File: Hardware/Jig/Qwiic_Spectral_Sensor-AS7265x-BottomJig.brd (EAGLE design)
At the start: 35.6 x 40.6 mm, 93 parts, among them J2 Serial Interface, J5 Flash Programming, J8 PTH, U1 AS72651, U3 4MB Flash, U5 AS72653, U6 AS72652

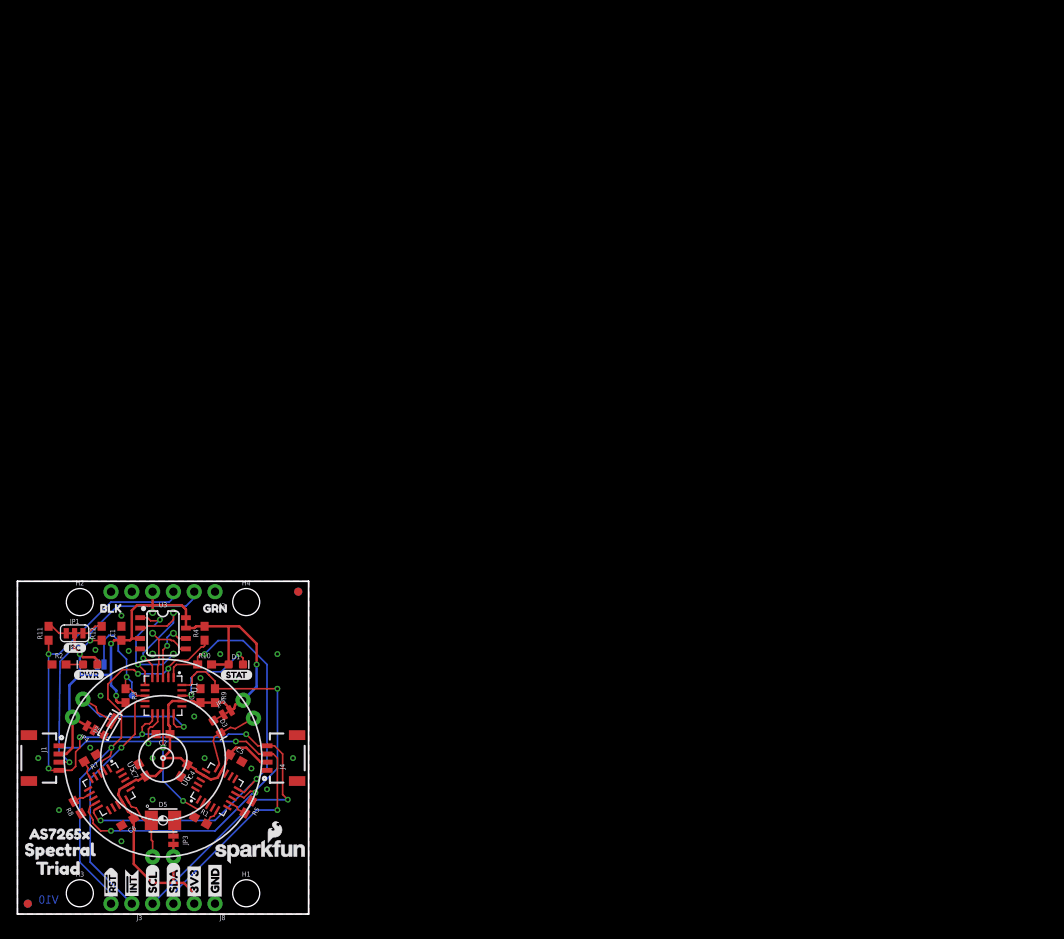
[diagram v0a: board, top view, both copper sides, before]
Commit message: Silk changes before panelization
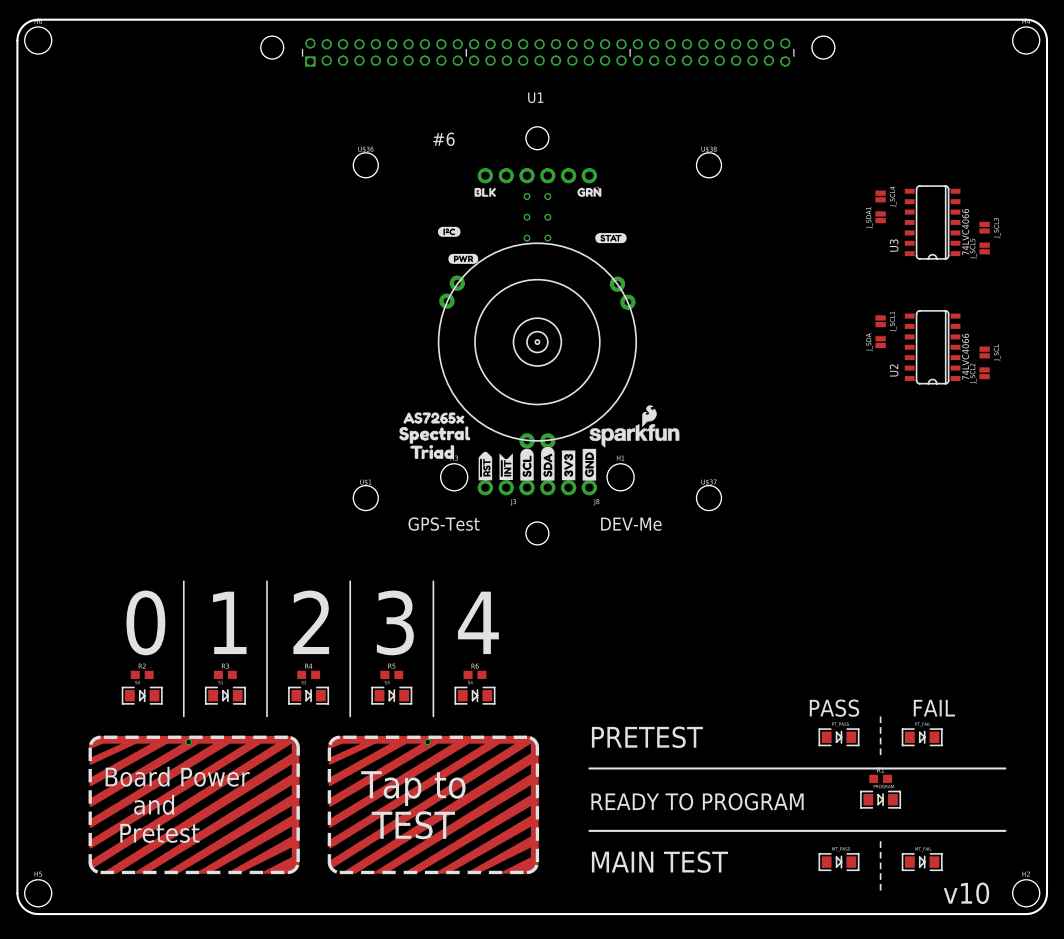
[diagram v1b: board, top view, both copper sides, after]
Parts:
- removed C1: 1.0uF, SparkFun-Capacitors:0603
- removed C2, C4, C6: 0.1uF, SparkFun-Capacitors:0603
- removed C3, C5, C7: 10uF, SparkFun-Capacitors:0603
- removed D1: BLUE, SparkFun-LED:LED-0603
- removed D2: 5700k, SparkFun-LED:SUPER_BRIGHT_SMD_LED_3014
- removed D3: IR, SparkFun-LED:LED-0603
- removed D4: RED, SparkFun-LED:LED-0603
- removed D5: UV, SparkFun-LED:PLCC-2
- removed FD1, FD2, FD3, FD4: FIDUCIAL1X2, SparkFun-Aesthetics:FIDUCIAL-1X2
- removed J1, J4: (no value), SparkFun-Connectors:1X04_1MM_RA
- removed JP1: (no value), SparkFun-Jumpers:SMT-JUMPER_3_2-NC_TRACE_SILK
- removed JP2: (no value), SparkFun-Jumpers:SMT-JUMPER_2_NO_SILK
- removed JP3, JP4, JP5: (no value), SparkFun-Jumpers:SMT-JUMPER_2_NC_TRACE_NO-SILK
- removed R10, R11, R12, R9: 2.2k, SparkFun-Resistors:0603
- removed R7, R8: 10k, SparkFun-Resistors:0603
- removed TP1: (no value), SparkFun-Connectors:PAD.03X.03
- removed U5: AS72653, Qwiic_Spectral_Sensor-AS7265x:LGA20
- removed U6: AS72652, Qwiic_Spectral_Sensor-AS7265x:LGA20
- added BUTTON1, BUTTON2: CAPSENSE_BUTTON_PAD_ONLY, Testing:CAPSENSE_BUTTON_PADS_ONLY
- added FRAME2: FRAME-LEDGER, SparkFun-Aesthetics:CREATIVE_COMMONS
- added H5, H6: STAND-OFF, SparkFun-Hardware:STAND-OFF
- added J_SCL, J_SCL3, J_SDA, J_SDA1: JUMPER-SMT_2_NO_NO-SILK, SparkFun-Jumpers:SMT-JUMPER_2_NO_NO-SILK
- added J_SCL1, J_SCL2, J_SCL4, J_SCL5: (no value), SparkFun-Jumpers:SMT-JUMPER_2_NO_NO-SILK
- added MT_FAIL, MT_PASS, PROGRAM, PT_FAIL, PT_PASS, S0, S1, S2, S3, S4: (no value), Testing:LED-1206
- added R6: 330, SparkFun-Resistors:0603
- added U2: 74LVC4066, Testing:SO14
- R1, R3, R4, R5: value 10k -> 330
- R2: value 1k -> 330
- U$1, U$36, U$37: device buzzard_labels (7):#0 -> SparkFun-Hardware:STAND-OFF-TIGHT
- U$38: device buzzard_labels (7):#1 -> SparkFun-Hardware:STAND-OFF-TIGHT
- U$39, U$40: device buzzard_labels (7):#1 -> SparkFun-Hardware:NUBBIN_LOCKER
- U1: value AS72651 -> FLYING_JALAPENO; device Qwiic_Spectral_Sensor-AS7265x:LGA20 -> Testing:FLYING_JALAPENO_V3_M
- U3: value 4MB Flash -> 74LVC4066; device SparkFun-IC-Memory:SO08 -> Testing:SO14
- moved H2 120.9 mm to (123.2, 2.54)
- moved H4 117.4 mm to (123.2, 106.7)
- moved U$38 108.9 mm to (84.5, 91.4), flipped to the top
- moved U3 106.2 mm to (111.8, 83.8), turned to 90 degrees
- moved U1 95.0 mm to (64.8, 109.2), turned to 0 degrees
- moved R1 83.2 mm to (105.4, 16.5), turned to 0 degrees
- moved U$40 78.1 mm to (63.5, 94.7), flipped to the top, turned to 0 degrees
- moved U$37 76.6 mm to (84.5, 50.8), flipped to the top
- moved U$36 74.8 mm to (42.5, 91.4), flipped to the top, turned to 0 degrees
- moved U$6 70.6 mm to (70.6, 77.5), turned to 240 degrees
- moved U$10 70.3 mm to (70.5, 82.5)
- moved BULB2 68.3 mm to (73.9, 75.8)
- moved BULB3 68.3 mm to (63.5, 57.8)
- moved H3 68.3 mm to (53.3, 53.3)
- moved J5 68.3 mm to (63.5, 85.1)
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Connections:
- removed net !RST-ADDR: U1.13, U6.2
- removed net I2C_ENB: JP2.2, R3.1, TP1.P$1, U1.8
- removed net N$1: D4.C, R2.2
- removed net N$11: D5.A, JP3.1
- removed net N$12: R8.2, U5.7
- removed net N$13: R7.2, U5.5
- removed net N$2: D1.C, U1.18
- removed net N$3: R5.2, U6.7
- removed net N$4: JP1.3, R12.2
- removed net N$5: JP1.1, R11.2
- removed net N$6: D2.A, JP4.1
- removed net N$8: D3.A, JP5.1
- removed net N$9: R1.2, U6.5
- removed net SCL_S: R9.1, U1.20, U5.9, U6.9
- removed net SDA_S: R10.1, U1.1, U5.10, U6.10
- new net 3.3V_POWER: U1.2, U1.32, U2.14, U3.14
- new net 5V_POWER: U1.3, U1.33
- new net JALAPENO_CS: J_SDA1.1, U1.60, U3.11
- new net JALAPENO_I2C_EN: U1.24, U2.13, U2.5
- new net JALAPENO_MISO: J_SCL5.1, U1.29, U3.1
- new net JALAPENO_MOSI: J_SCL3.1, U1.59, U3.4
- new net JALAPENO_RX1-I: J_SDA.1, U1.52, U2.11
- new net JALAPENO_SCK: J_SCL4.1, U1.30, U3.8
- new net JALAPENO_SCL: J_SCL.1, U1.53, U2.4
- new net JALAPENO_SDA: J_SCL2.1, U1.23, U2.1
- new net JALAPENO_SERIAL_EN: U1.54, U2.12, U2.6
- new net JALAPENO_SPI_EN: U3.12, U3.13, U3.5, U3.6
- new net JALAPENO_TX1-O: J_SCL1.1, U1.22, U2.8
- new net J_24: U1.25
- new net J_25: U1.55
- new net J_26: U1.26
- new net J_27: U1.56
- new net J_28: U1.27
- new net J_29: U1.57
- new net J_30: U1.28
- new net J_A0: U1.37
- new net J_A1: U1.8
- new net J_A2: U1.38
- new net J_A3: U1.9
- new net J_A4: U1.39
- new net J_PWM2: U1.14
- new net J_PWM3: U1.44
- new net J_PWM4: U1.15
- new net J_PWM5: U1.45
- new net N$10: PT_FAIL.A, U1.36
- new net N$14: MT_PASS.A, U1.6
- new net N$15: MT_FAIL.A, U1.35
- new net N$16: BUTTON2.CAPSENSE_PAD, U1.58
- new net N$17: BUTTON1.CAPSENSE_PAD, U1.5
- new net N$18: R1.2, U1.19
- new net N$19: PROGRAM.A, R1.1
- new net N$20: R6.2, U1.46
- new net N$21: R5.2, U1.17
- new net N$22: R4.2, U1.47
- new net N$23: R3.2, U1.18
- new net N$24: R2.2, U1.48
- new net N$25: R6.1, S4.A
- new net N$26: R5.1, S3.A
- new net N$27: R4.1, S2.A
- new net N$28: R3.1, S1.A
- new net N$29: R2.1, S0.A
- new net N$7: PT_PASS.A, U1.7
- new net TARGET_CS: J_SDA1.2, U3.10
- new net TARGET_MISO: J_SCL5.2, U3.2
- new net TARGET_MOSI: J_SCL3.2, U3.3
- new net TARGET_RX: J_SCL1.2, U2.9
- new net TARGET_SCK: J_SCL4.2, U3.9
- new net TARGET_SCL: J_SCL.2, U2.3
- new net TARGET_SDA: J_SCL2.2, U2.2
- new net TARGET_TX: J_SDA.2, U2.10
- net !CS_EE: no longer U1.6, U3.1
- net !INT: no longer U1.9
- net !RST: no longer R4.1, U1.2, U5.2
- net 3.3V: no longer C1.1, C2.1, C3.1, C4.1, C5.1, C6.1, C7.1, D1.A, D4.A, J1.2, J4.2, JP1.2, JP3.2, JP4.2, JP5.2, R10.2, R3.2, R4.2, R9.2, U1.14, U1.17, U3.3, U3.7, U3.8, U5.14, U5.17, U6.14, U6.17
- net GND: now also MT_FAIL.C, MT_PASS.C, PROGRAM.C, PT_FAIL.C, PT_PASS.C, S0.C, S1.C, S2.C, S3.C, S4.C, U1.1, U1.31, U2.7, U3.7; no longer C1.2, C2.2, C3.2, C4.2, C5.2, C6.2, C7.2, J1.1, J4.1, JP2.1, R1.1, R2.1, R5.1, R7.1, R8.1, U1.16, U3.4, U5.16, U6.16
- net LED_DRV: no longer D2.C, U1.15
- net LED_DRV1: no longer D3.C, U6.15
- net LED_DRV2: no longer D5.C, U5.15
- net MISO: no longer U1.5, U3.2
- net MOSI: no longer U1.4, U3.5
- net RX/SCL: no longer J1.4, J4.4, R11.1, U1.11
- net SCK: no longer U1.3, U3.6
- net TX/SDA: no longer J1.3, J4.3, R12.1, U1.12
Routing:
- net 3.3V: track 143.3 -> 0.00 mm, vias 4 -> 0
- net RX/SCL: track 99.0 -> 0.00 mm, vias 6 -> 0
- net TX/SDA: track 93.2 -> 0.00 mm, vias 5 -> 0
- net SDA_S: track 56.9 -> 0.00 mm, vias 3 -> 0
- net SCL_S: track 56.2 -> 0.00 mm, vias 3 -> 0
- net !RST: track 50.8 -> 0.00 mm, vias 3 -> 0
- net !INT: track 30.2 -> 0.00 mm, vias 1 -> 0
- net LED_DRV: track 21.0 -> 0.00 mm, vias 1 -> 0
- net !CS_EE: track 17.6 -> 0.00 mm, vias 2 -> 0
- net I2C_ENB: track 16.8 -> 0.00 mm, vias 1 -> 0
- net MISO: track 15.5 -> 0.00 mm, vias 1 -> 0
- net !RST-ADDR: track 14.9 -> 0.00 mm, vias 2 -> 0
- net N$2: track 11.8 -> 0.00 mm, vias 2 -> 0
- net MOSI: track 9.65 -> 0.00 mm
- net LED_DRV1: track 9.51 -> 0.00 mm
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- removed copper zone on layer 1, net GND
- removed copper zone on layer 16, net GND
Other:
- board size 35.6 x 40.6 mm -> 125.7 x 109.2 mm
- board text added: "#6"
- board text added: "0"
- board text added: "1"
- board text added: "2"
- board text added: "3"
- board text added: "4"
- board text added: "Board Power and Pretest"
- board text added: "DEV-Me"
- board text added: "FAIL"
- board text added: "GPS-Test"
- board text added: "MAIN TEST"
- board text added: "PASS"
- board text added: "PRETEST"
- board text added: "READY TO PROGRAM"
- board text added: "Tap to TEST"
- board text added: "v10"
- board text removed: "V10"
